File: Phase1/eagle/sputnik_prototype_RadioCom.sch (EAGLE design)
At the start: 74 parts, among them X2 332-22, Y1 32MHz

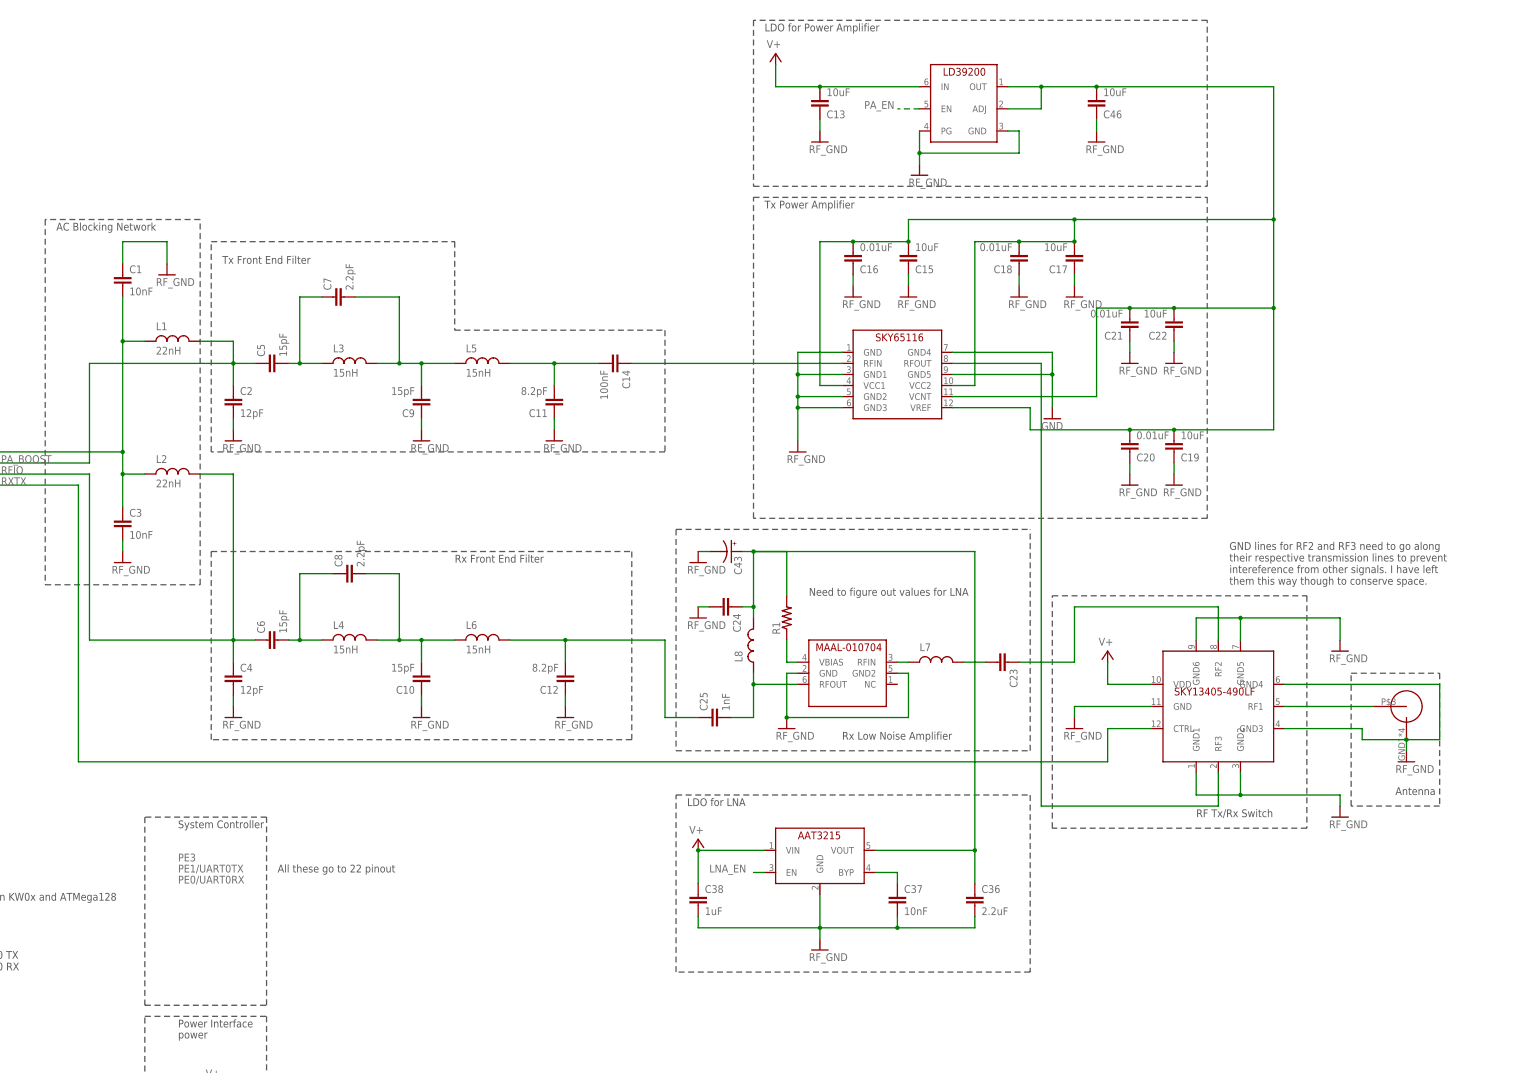
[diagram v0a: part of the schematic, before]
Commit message: fixed symbols
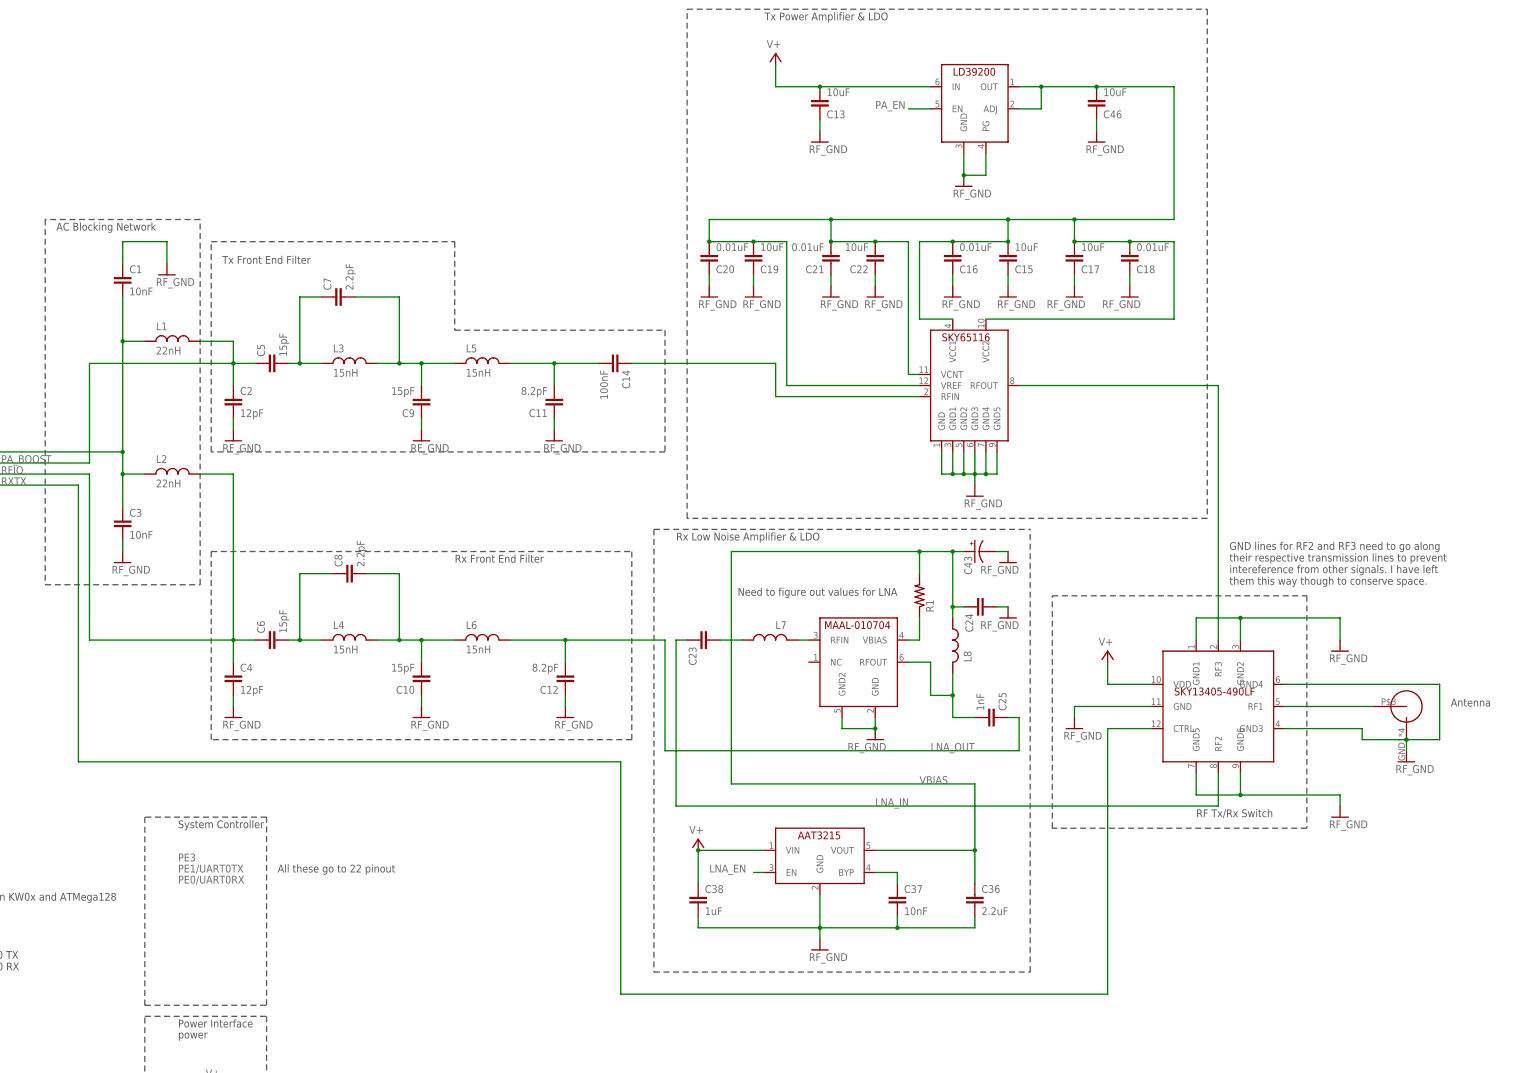
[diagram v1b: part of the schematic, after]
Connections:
- net N$20 renamed LNA_OUT
- net N$5 renamed LNA_IN
- removed net N$2 (its old number): C24.1, C43.+, L8.2, R1.2
- removed net N$9: C36.1, U$7.VOUT
- new net VBIAS: C24.1, C36.1, C43.+, L8.2, R1.2, U$7.VOUT
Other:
- note added: "Rx Low Noise Amplifier & LDO"
- note added: "Tx Power Amplifier & LDO"
- note removed: "LDO for LNA"
- note removed: "LDO for Power Amplifier"
- note removed: "Rx Low Noise Amplifier"
- note removed: "Tx Power Amplifier"
- moved on the sheet: C15, C16, C18, C19, C20, C21, C22, C23, C24, C25, C43, L7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
